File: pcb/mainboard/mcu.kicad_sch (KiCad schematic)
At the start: 54 parts, among them Y100 24MHz, Y101 32.768K

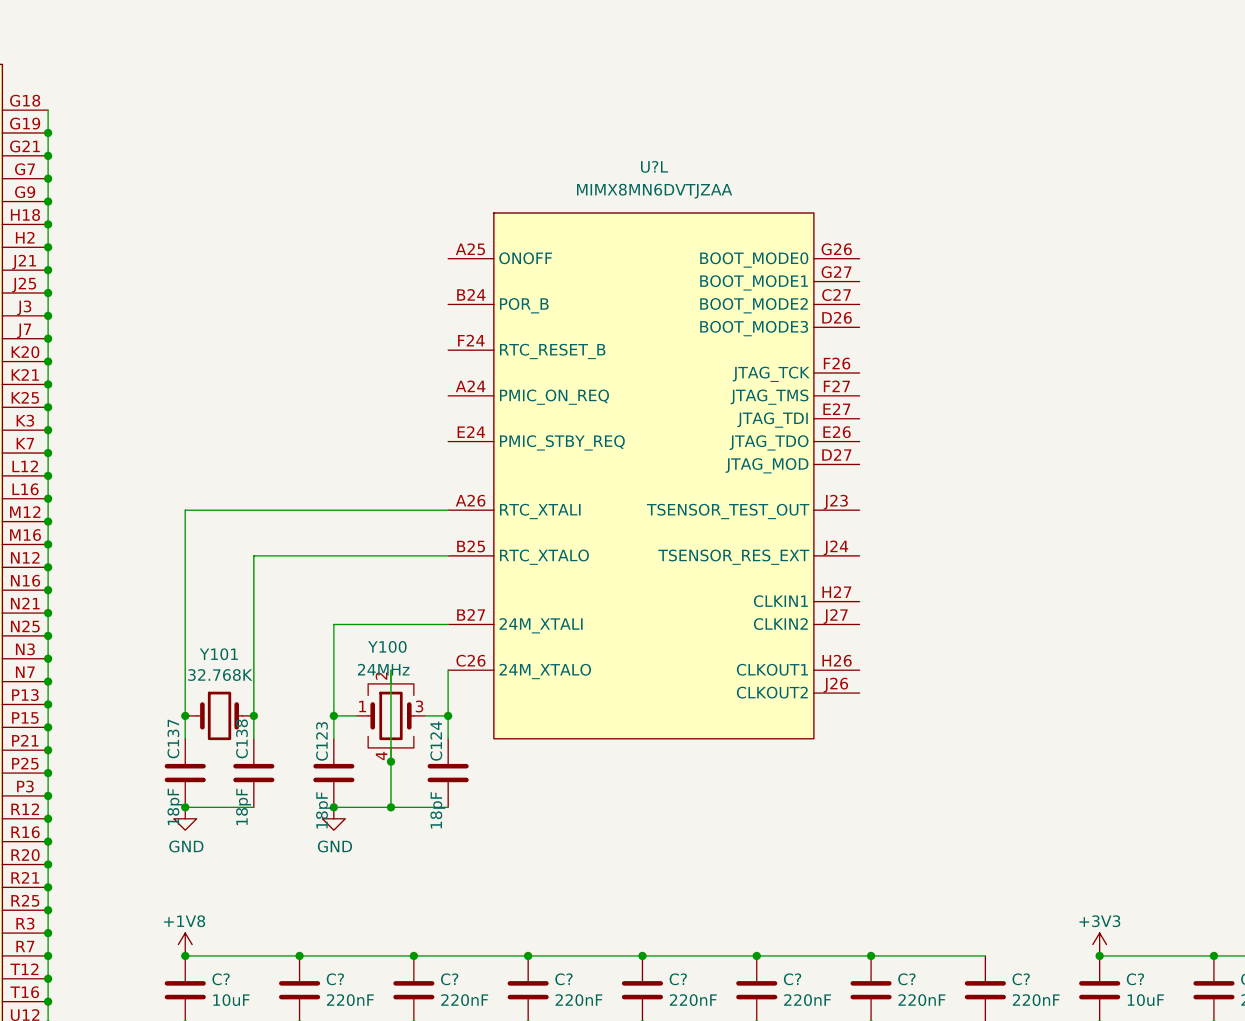
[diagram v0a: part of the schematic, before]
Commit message: Working on mainboard schematics
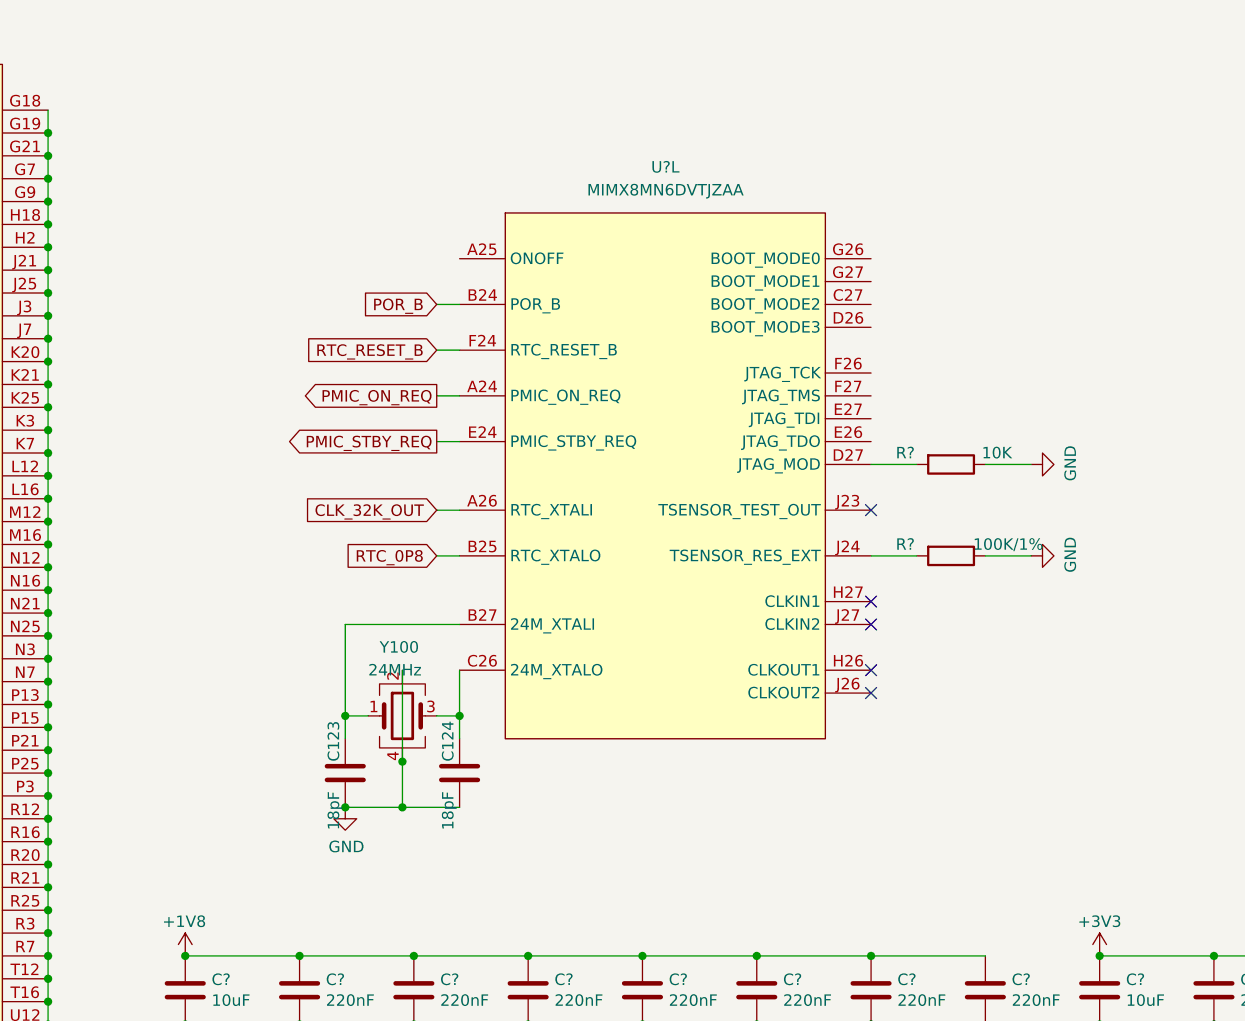
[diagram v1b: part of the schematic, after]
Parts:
- removed C137, C138: 18pF, Capacitor_SMD:C_0402_1005Metric, symbol Device:C
- removed Y101: 32.768K, Crystal:Crystal_SMD_TXC_9HT11-2Pin_2.0x1.2mm_HandSoldering, symbol Device:Crystal
- added R?: 100K/1%, Resistor_SMD:R_0402_1005Metric, symbol Device:R
- added R?: 10K, Resistor_SMD:R_0402_1005Metric, symbol Device:R
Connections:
- net GND: now also R?.1, R?.1
- net RTC_0P8: now also U?.B25 (RTC_XTALO)
- net PMIC_ON_REQ: now reaches U?.A24 (PMIC_ON_REQ)
- net CLK_32K_OUT: now reaches U?.A26 (RTC_XTALI)
- net POR_B: now reaches U?.B24 (POR_B)
- net at U?.D27 (JTAG_MOD): now also R?.2
- net PMIC_STBY_REQ: now reaches U?.E24 (PMIC_STBY_REQ)
- net RTC_RESET_B: now reaches U?.F24 (RTC_RESET_B)
- net at U?.J24 (TSENSOR_RES_EXT): now also R?.2
- no-connect marks 12 -> 17
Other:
- moved on the sheet: C123, C124, U?L, Y100
